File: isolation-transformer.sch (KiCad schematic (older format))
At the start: 0 parts

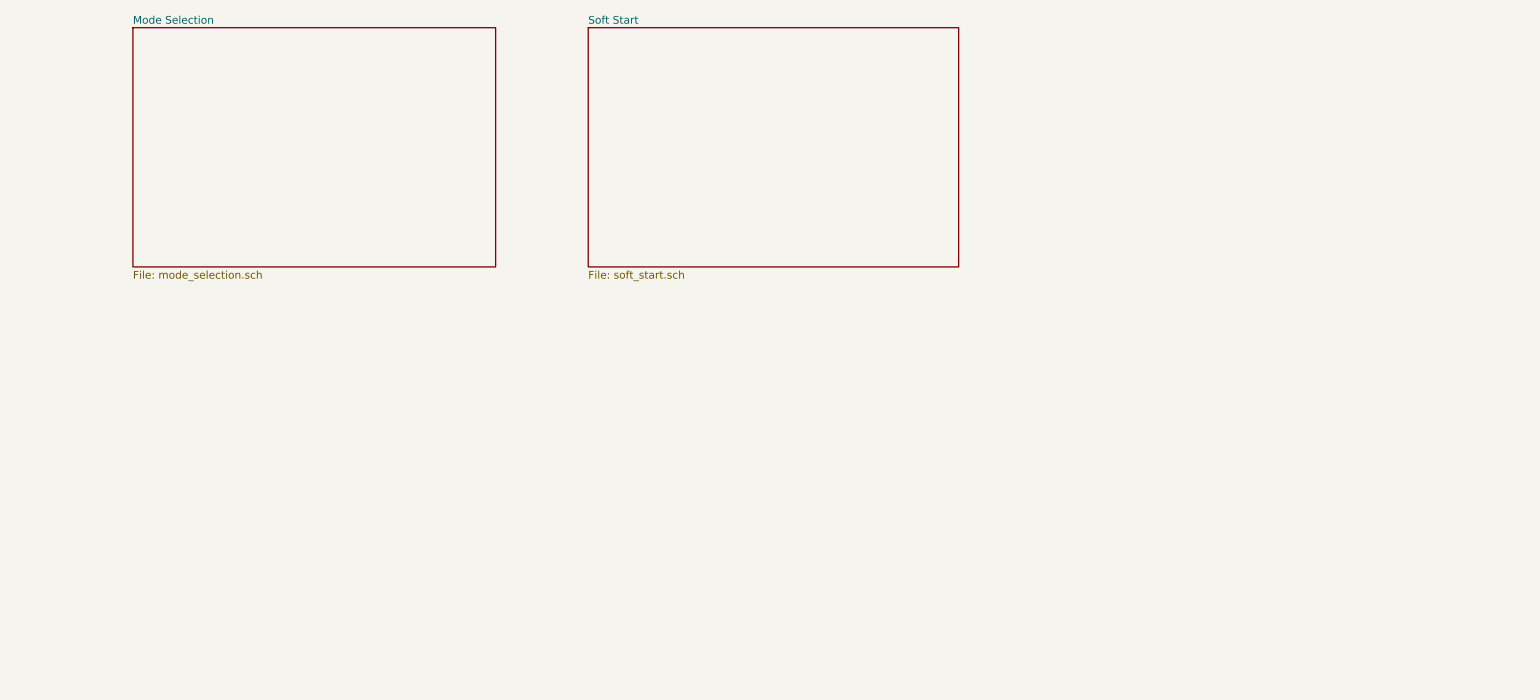
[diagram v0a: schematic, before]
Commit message: Final schematic version
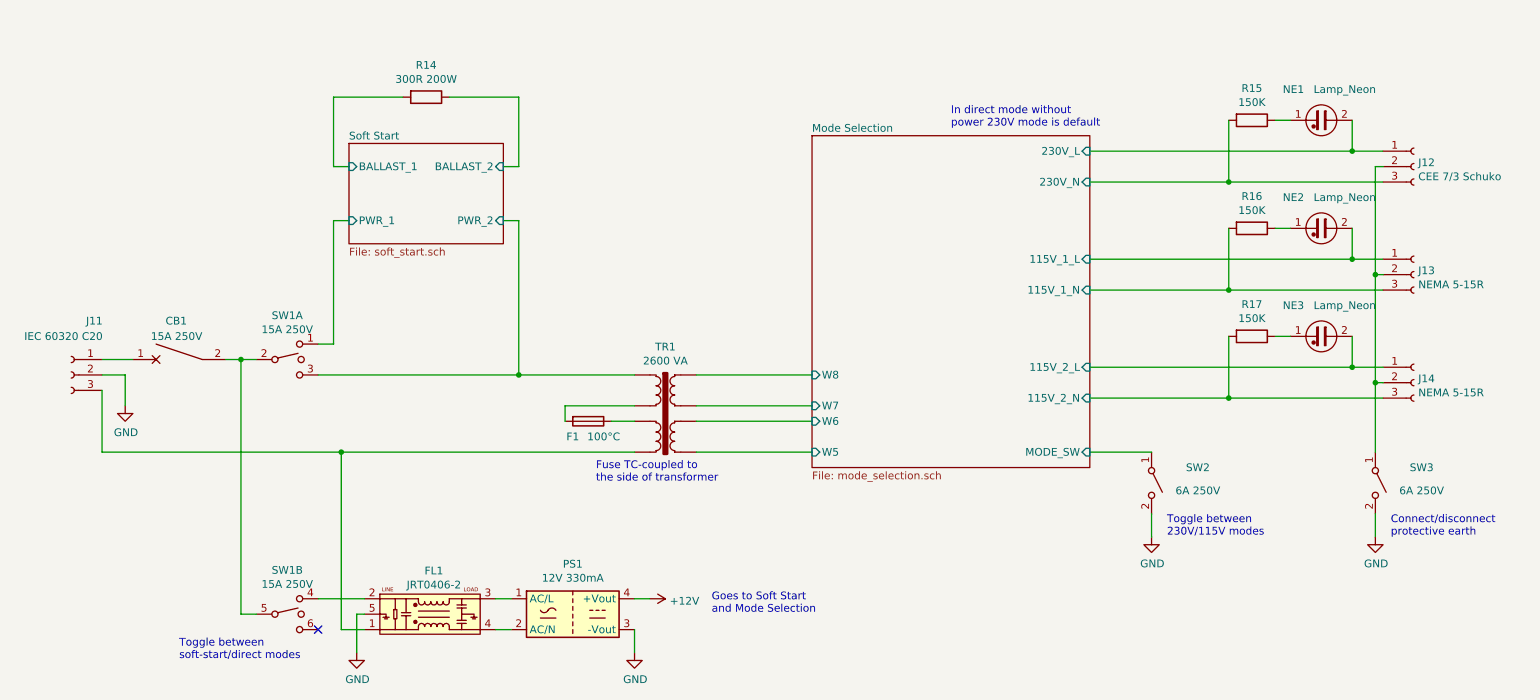
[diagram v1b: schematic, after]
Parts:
- added CB1: 15A 250V, symbol Device:CircuitBreaker_1P
- added F1: 100°C, symbol Device:Fuse
- added FL1: JRT0406-2, symbol CustomParts:EMI_Filter_LL_CCC
- added J11: IEC 60320 C20, symbol Connector:Conn_01x03_Female
- added J12: CEE 7/3 Schuko, symbol Connector:Conn_01x03_Female
- added J13, J14: NEMA 5-15R, symbol Connector:Conn_01x03_Female
- added NE1, NE2, NE3: Lamp_Neon, symbol Device:Lamp_Neon
- added PS1: 12V 330mA, symbol Converter_ACDC:HLK-PM12
- added R14: 300R 200W, symbol Device:R
- added R15, R16, R17: 150K, symbol Device:R
- added SW1: 15A 250V, symbol CustomParts:SW_DPDT_x2_MSM
- added SW2, SW3: 6A 250V, symbol Switch:SW_SPST
- added TR1: 2600 VA, symbol Transformer:TRANSF6
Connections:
- new net: F1.2, TR1.2
- new net: F1.1, TR1.3
- new net: FL1.1, J11.3 (Pin_3), TR1.4
- new net: CB1.1, J11.1 (Pin_1)
- new net: CB1.2, SW1.2 (B), SW1.5 (B)
- new net: NE1.1, R15.1
- new net: FL1.3, PS1.1 (AC/L)
- new net: FL1.4, PS1.2 (AC/N)
- new net: FL1.2, SW1.4 (A)
- new net: J12.2 (Pin_2), J13.2 (Pin_2), J14.2 (Pin_2), SW3.1 (A)
- new net: NE2.1, R16.1
- new net: NE3.1, R17.1
- new net +12V: PS1.4 (+Vout)
- new net GND: FL1.5, J11.2 (Pin_2), PS1.3 (-Vout), SW2.2 (B), SW3.2 (B)
- new net Mode Selection/115V_1_L: J13.1 (Pin_1), NE2.2
- new net Mode Selection/115V_1_N: J13.3 (Pin_3), R16.2
- new net Mode Selection/115V_2_L: J14.1 (Pin_1), NE3.2
- new net Mode Selection/115V_2_N: J14.3 (Pin_3), R17.2
- new net Mode Selection/230V_L: J12.1 (Pin_1), NE1.2
- new net Mode Selection/230V_N: J12.3 (Pin_3), R15.2
- new net Mode Selection/MODE_SW: SW2.1 (A)
- new net Mode Selection/W5: TR1.5
- new net Mode Selection/W6: TR1.6
- new net Mode Selection/W7: TR1.7
- new net Mode Selection/W8: TR1.8
- new net Soft Start/BALLAST_1: R14.2
- new net Soft Start/BALLAST_2: R14.1
- new net Soft Start/PWR_1: SW1.1 (A)
- new net Soft Start/PWR_2: SW1.3 (C), TR1.1
- no-connect marks 0 -> 1
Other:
- note added: "Connect/disconnect\nprotective earth"
- note added: "Fuse TC-coupled to\nthe side of transformer"
- note added: "Goes to Soft Start\nand Mode Selection"
- note added: "In direct mode without\npower 230V mode is default"
- note added: "Toggle between\n230V/115V modes"
- note added: "Toggle between\nsoft-start/direct modes"
